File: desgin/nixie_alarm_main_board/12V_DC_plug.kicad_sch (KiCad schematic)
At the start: 4 parts, among them J1 DCPLUG 2x6.4mm 2A

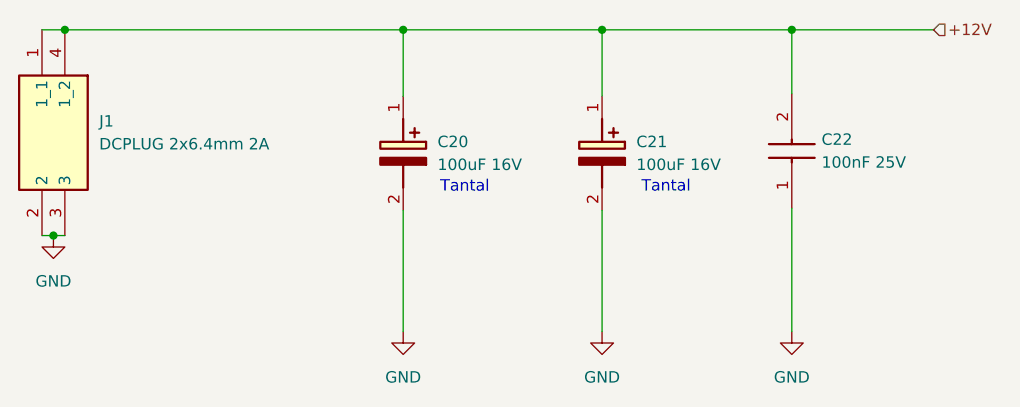
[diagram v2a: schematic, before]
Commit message: new board v1
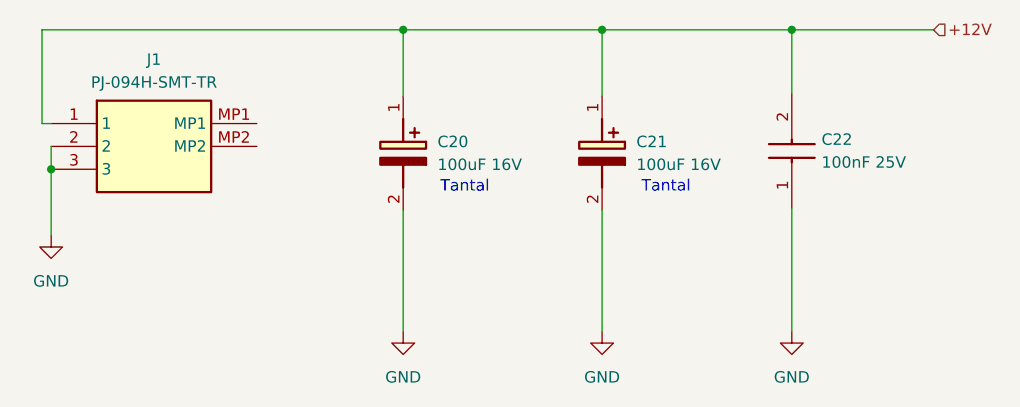
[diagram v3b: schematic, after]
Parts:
- removed J1: DCPLUG 2x6.4mm 2A, DCJ20005AK1A, symbol SamacSys_Parts:DCJ200-05-A-K1-A
- added J1: PJ-094H-SMT-TR, PJ094HSMTTR, symbol SamacSys_Parts:PJ-094H-SMT-TR
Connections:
- net +12V: now also J1.1
- net GND: now also J1.2, J1.3
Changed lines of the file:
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@@
-	)
-	(junction
-		(at 104.14 93.472)
-		(diameter 0)
-		(color 0 0 0 0)
 	)
 	(junction
@@
 	)
 	(junction
-		(at 105.41 70.612)
+		(at 103.886 86.106)
 		(diameter 0)
 		(color 0 0 0 0)
@@
 	(wire
 		(pts
+			(xy 102.87 70.612) (xy 102.87 81.026)
+		)
+		(stroke
+			(width 0)
+			(type default)
+		)
+	)
+	(wire
+		(pts
 			(xy 143.002 70.612) (xy 143.002 77.978)
 		)
@@
 	(wire
 		(pts
-			(xy 102.87 70.612) (xy 105.41 70.612)
-		)
-		(stroke
-			(width 0)
-			(type default)
-		)
-	)
-	(wire
-		(pts
-			(xy 105.41 70.612) (xy 143.002 70.612)
+			(xy 102.87 70.612) (xy 143.002 70.612)
+		)
+		(stroke
+			(width 0)
+			(type default)
+		)
+	)
+	(wire
+		(pts
+			(xy 102.87 81.026) (xy 103.886 81.026)
 		)
 		(stroke
@@
 	(wire
 		(pts
-			(xy 104.14 93.472) (xy 105.41 93.472)
+			(xy 103.886 83.566) (xy 103.886 86.106)
 		)
 		(stroke
@@
 	(wire
 		(pts
+			(xy 103.886 86.106) (xy 103.886 93.472)
+		)
+		(stroke
+			(width 0)
+			(type default)
+		)
+	)
+	(wire
+		(pts
 			(xy 165.1 70.612) (xy 143.002 70.612)
 		)
@@
 		(pts
 			(xy 186.182 90.424) (xy 186.182 104.14)
-		)
-		(stroke
-			(width 0)
-			(type default)
-		)
-	)
-	(wire
-		(pts
-			(xy 102.87 93.472) (xy 104.14 93.472)
 		)
 		(stroke
@@
 	)
 	(symbol
-		(lib_id "SamacSys_Parts:DCJ200-05-A-K1-A")
-		(at 105.41 70.612 270)
-		(unit 1)
-		(exclude_from_sim no)
-		(in_bom yes)
-		(on_board yes)
-		(dnp no)
-		(fields_autoplaced yes)
-		(property "Reference" "J1"
-			(at 109.22 80.7719 90)
-			(effects
-				(font
-					(size 1.27 1.27)
-				)
-				(justify left)
-			)
-		)
-		(property "Value" "DCPLUG 2x6.4mm 2A"
-			(at 109.22 83.3119 90)
-			(effects
-				(font
-					(size 1.27 1.27)
-				)
-				(justify left)
-			)
-		)
-		(property "Footprint" "DCJ20005AK1A"
-			(at 10.49 89.662 0)
-			(effects
-				(font
-					(size 1.27 1.27)
-				)
-				(justify left top)
-				(hide yes)
-			)
-		)
-		(property "Datasheet" "https://componentsearchengine.com/Datasheets/2/DCJ200-05-A-K1-A.pdf"
-			(at -89.51 89.662 0)
-			(effects
-				(font
-					(size 1.27 1.27)
-				)
-				(justify left top)
-				(hide yes)
-			)
-		)
-		(property "Description" "DCJ200 Series 20 V 5 A 2 Conductors/3 Contacts Horizontal SMT DC Power Jack"
-			(at 105.41 70.612 0)
-			(effects
-				(font
-					(size 1.27 1.27)
-				)
-				(hide yes)
-			)
-		)
-		(property "Height" "11.3"
-			(at -289.51 89.662 0)
-			(effects
-				(font
-					(size 1.27 1.27)
-				)
-				(justify left top)
-				(hide yes)
-			)
-		)
-		(property "Mouser Part Number" "640-DCJ200-05-A-K1-A"
-			(at -389.51 89.662 0)
-			(effects
-				(font
-					(size 1.27 1.27)
-				)
-				(justify left top)
-				(hide yes)
-			)
-		)
-		(property "Mouser Price/Stock" "https://www.mouser.co.uk/ProductDetail/GCT/DCJ200-05-A-K1-A?qs=KUoIvG%2F9IlZdgC%252BD5EAHVw%3D%3D"
-			(at -489.51 89.662 0)
-			(effects
-				(font
-					(size 1.27 1.27)
-				)
-				(justify left top)
-				(hide yes)
-			)
-		)
-		(property "Manufacturer_Name" "GCT (GLOBAL CONNECTOR TECHNOLOGY)"
-			(at -589.51 89.662 0)
-			(effects
-				(font
-					(size 1.27 1.27)
-				)
-				(justify left top)
-				(hide yes)
-			)
-		)
-		(property "Manufacturer_Part_Number" "DCJ200-05-A-K1-A"
-			(at -689.51 89.662 0)
-			(effects
-				(font
-					(size 1.27 1.27)
-				)
-				(justify left top)
-				(hide yes)
-			)
-		)
-		(pin "2"
-		)
-		(pin "4"
-		)
-		(pin "3"
-		)
-		(pin "1"
-		)
-		(instances
-			(project "nixie_alarm_main_board"
-				(path "/a0d555d7-39a0-4a98-b831-70d97d0aa5a1/3f162d9f-7cb0-459b-831b-ac42fb433594"
-					(reference "J1")
-					(unit 1)
-				)
-			)
-		)
-	)
-	(symbol
 		(lib_id "power:GND")
 		(at 186.182 104.14 0)
@@
 	)
 	(symbol
+		(lib_id "SamacSys_Parts:PJ-094H-SMT-TR")
+		(at 103.886 81.026 0)
+		(unit 1)
+		(exclude_from_sim no)
+		(in_bom yes)
+		(on_board yes)
+		(dnp no)
+		(fields_autoplaced yes)
+		(property "Reference" "J1"
+			(at 115.316 73.914 0)
+			(effects
+				(font
+					(size 1.27 1.27)
+				)
+			)
+		)
+		(property "Value" "PJ-094H-SMT-TR"
+			(at 115.316 76.454 0)
+			(effects
+				(font
+					(size 1.27 1.27)
+				)
+			)
+		)
+		(property "Footprint" "PJ094HSMTTR"
+			(at 122.936 175.946 0)
+			(effects
+				(font
+					(size 1.27 1.27)
+				)
+				(justify left top)
+				(hide yes)
+			)
+		)
+		(property "Datasheet" "https://www.cuidevices.com/product/resource/digikeypdf/pj-094h-smt-tr.pdf"
+			(at 122.936 275.946 0)
+			(effects
+				(font
+					(size 1.27 1.27)
+				)
+				(justify left top)
+				(hide yes)
+			)
+		)
+		(property "Description" "DC Power Connectors power jack, 0.65 x 2.75 mm, horizontal, SMT, high current, 1 switch, w/ shielding, T&R package"
+			(at 103.886 81.026 0)
+			(effects
+				(font
+					(size 1.27 1.27)
+				)
+				(hide yes)
+			)
+		)
+		(property "Height" "3.7"
+			(at 122.936 475.946 0)
+			(effects
+				(font
+					(size 1.27 1.27)
+				)
+				(justify left top)
+				(hide yes)
+			)
+		)
+		(property "Mouser Part Number" "490-PJ-094H-SMT-TR"
+			(at 122.936 575.946 0)
+			(effects
+				(font
+					(size 1.27 1.27)
+				)
+				(justify left top)
+				(hide yes)
+			)
+		)
+		(property "Mouser Price/Stock" "https://www.mouser.co.uk/ProductDetail/CUI-Devices/PJ-094H-SMT-TR?qs=l7cgNqFNU1iCmsfPShkP7A%3D%3D"
+			(at 122.936 675.946 0)
+			(effects
+				(font
+					(size 1.27 1.27)
+				)
+				(justify left top)
+				(hide yes)
+			)
+		)
+		(property "Manufacturer_Name" "Same Sky"
+			(at 122.936 775.946 0)
+			(effects
+				(font
+					(size 1.27 1.27)
+				)
+				(justify left top)
+				(hide yes)
+			)
+		)
+		(property "Manufacturer_Part_Number" "PJ-094H-SMT-TR"
+			(at 122.936 875.946 0)
+			(effects
+				(font
+					(size 1.27 1.27)
+				)
+				(justify left top)
+				(hide yes)
+			)
+		)
+		(pin "1"
+		)
+		(pin "2"
+		)
+		(pin "MP1"
+		)
+		(pin "3"
+		)
+		(pin "MP2"
+		)
+		(instances
+			(project "nixie_alarm_main_board"
+				(path "/a0d555d7-39a0-4a98-b831-70d97d0aa5a1/3f162d9f-7cb0-459b-831b-ac42fb433594"
+					(reference "J1")
+					(unit 1)
+				)
+			)
+		)
+	)
+	(symbol
 		(lib_id "power:GND")
 		(at 143.002 104.14 0)
@@
 	(symbol
 		(lib_id "power:GND")
-		(at 104.14 93.472 0)
+		(at 103.886 93.472 0)
 		(unit 1)
 		(exclude_from_sim no)
@@
 		(fields_autoplaced yes)
 		(property "Reference" "#PWR050"
-			(at 104.14 99.822 0)
+			(at 103.886 99.822 0)
 			(effects
 				(font
@@
 		)
 		(property "Value" "GND"
-			(at 104.14 98.552 0)
+			(at 103.886 98.552 0)
 			(effects
 				(font
@@
 		)
 		(property "Footprint" ""
-			(at 104.14 93.472 0)
+			(at 103.886 93.472 0)
 			(effects
 				(font
@@
 		)
 		(property "Datasheet" ""
-			(at 104.14 93.472 0)
+			(at 103.886 93.472 0)
 			(effects
 				(font
@@
 		)
 		(property "Description" "Power symbol creates a global label with name \"GND\" , ground"
-			(at 104.14 93.472 0)
-			(effects
-				(font
+			(at 103.886 93.472 0)
+			(effects
+				(font
